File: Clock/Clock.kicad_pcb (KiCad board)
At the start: 2 copper layers, 85 x 99 mm, 50 parts, among them J1 LED, J2 BUS LEDs, J3 USB_B_Micro, SW1 Pulse, SW2 SW_SPDT, SW3 Reset, U1 TLC555xP, U2 TLC555xP, U3 TLC555xP, U4 74HC14, U5 74LS08, U6 74LS32

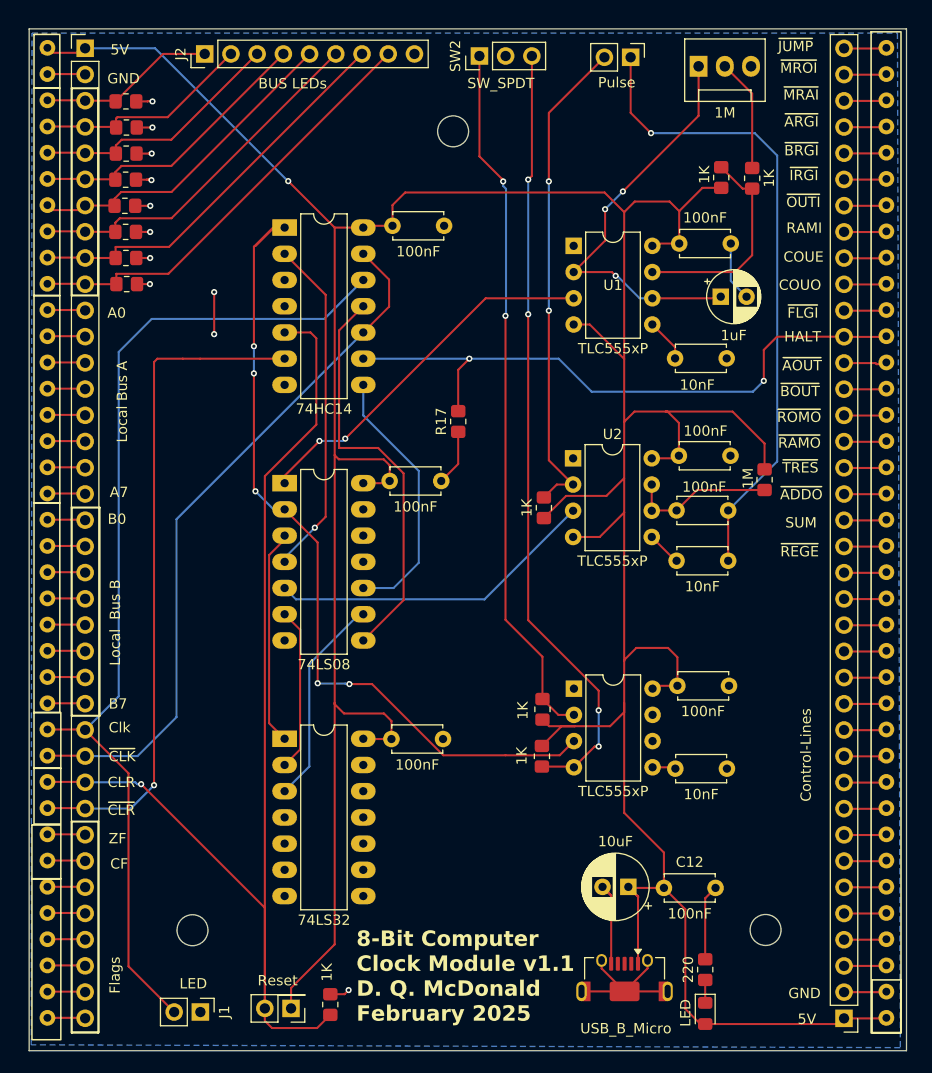
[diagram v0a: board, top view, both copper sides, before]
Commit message: Updated to v2.0. Sent to manufacturing after review.
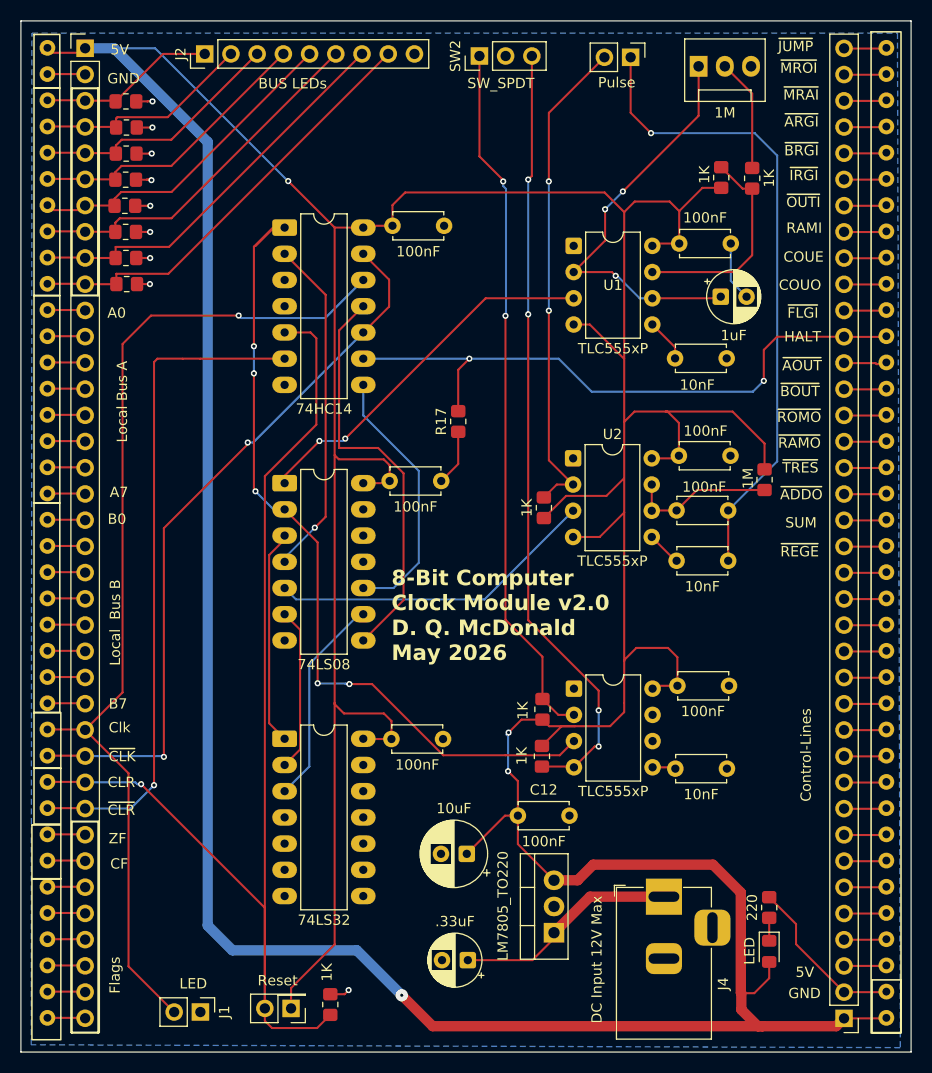
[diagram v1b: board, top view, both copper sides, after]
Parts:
- removed J3: USB_B_Micro, Connector_USB:USB_Micro-AB_Molex_47590-0001
- removed REF** (x3): MountingHole_3mm, MountingHole:MountingHole_3mm
- added C14: .33uF, Capacitor_THT:CP_Radial_D5.0mm_P2.50mm, F.Cu at (66.3, 119.7)
- added J4: DC Input 12V Max, Connector_BarrelJack:BarrelJack_Horizontal, F.Cu at (85.3, 113.5)
- added U7: LM7805_TO220, Package_TO_SOT_THT:TO-220-3_Vertical, F.Cu at (74.7, 117.0)
- moved C11 16.0 mm to (66.2, 109.3)
- moved C12 15.8 mm to (71.2, 105.7)
- moved D1 8.64 mm to (95.5, 118.8)
- moved R16 8.64 mm to (95.5, 114.5)
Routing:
- net 5V: track 368.5 -> 531.1 mm, vias 1 -> 4
- net Net-(U7-VI): track 0.00 -> 21.9 mm
- net unconnected-(J3-Shield-Pad6)_1: track 15.3 -> 0.00 mm
- net GND: track 118.3 -> 110.0 mm, vias 12 -> 10
- net ~{CLOCK}: track 68.8 -> 70.5 mm, vias 0 -> 2
- net CLOCK: track 99.4 -> 99.8 mm, vias 0 -> 1
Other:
- board size 85 x 99 mm -> 86.2 x 99.9 mm
- board text added: "8-Bit Computer Clock Module v2.0 D. Q. McDonald May 2026"
- board text removed: "8-Bit Computer Clock Module v1.1 D. Q. McDonald February 2025"
